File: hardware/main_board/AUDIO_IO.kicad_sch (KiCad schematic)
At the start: 10 parts, among them IC501 LM4890M_NOPB, J501 Conn_01x03_Pin, J502 AudioJack

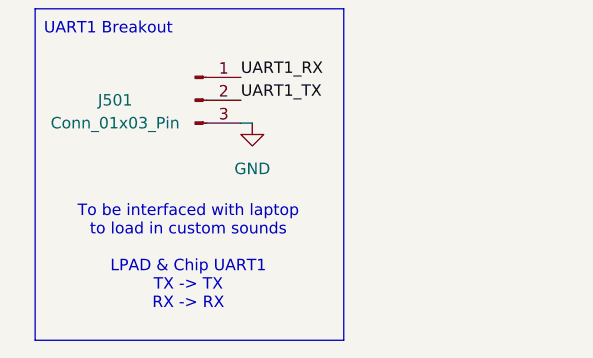
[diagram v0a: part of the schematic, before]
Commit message: pcb review changes
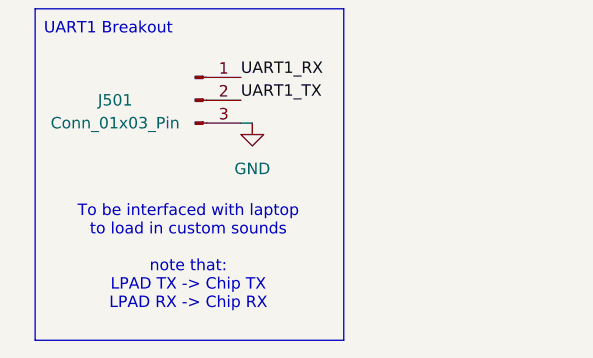
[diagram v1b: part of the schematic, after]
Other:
- note added: "To be interfaced with laptop to load in custom sounds note that: LPAD TX -> Chip TX LPAD RX -> Chip RX"
- note removed: "To be interfaced with laptop to load in custom sounds LPAD & Chip UART1 TX -> TX RX -> RX"
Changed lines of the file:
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@@
 		)
 	)
-	(text "To be interfaced with laptop\nto load in custom sounds\n\nLPAD & Chip UART1 \nTX -> TX\nRX -> RX"
+	(text "To be interfaced with laptop\nto load in custom sounds\n\nnote that: \nLPAD TX -> Chip TX\nLPAD RX -> Chip RX"
 		(exclude_from_sim no)
 		(at 30.988 116.586 0)
